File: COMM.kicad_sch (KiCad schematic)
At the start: 14 parts, among them J1 SMA Conn. (RFPC-SMA29-F), SW1 Inhibit Switch (SS5GLD2), U1 AX.25 Module (DMR818SU), U2 XBee Module (XBP9B-DMSTB002)

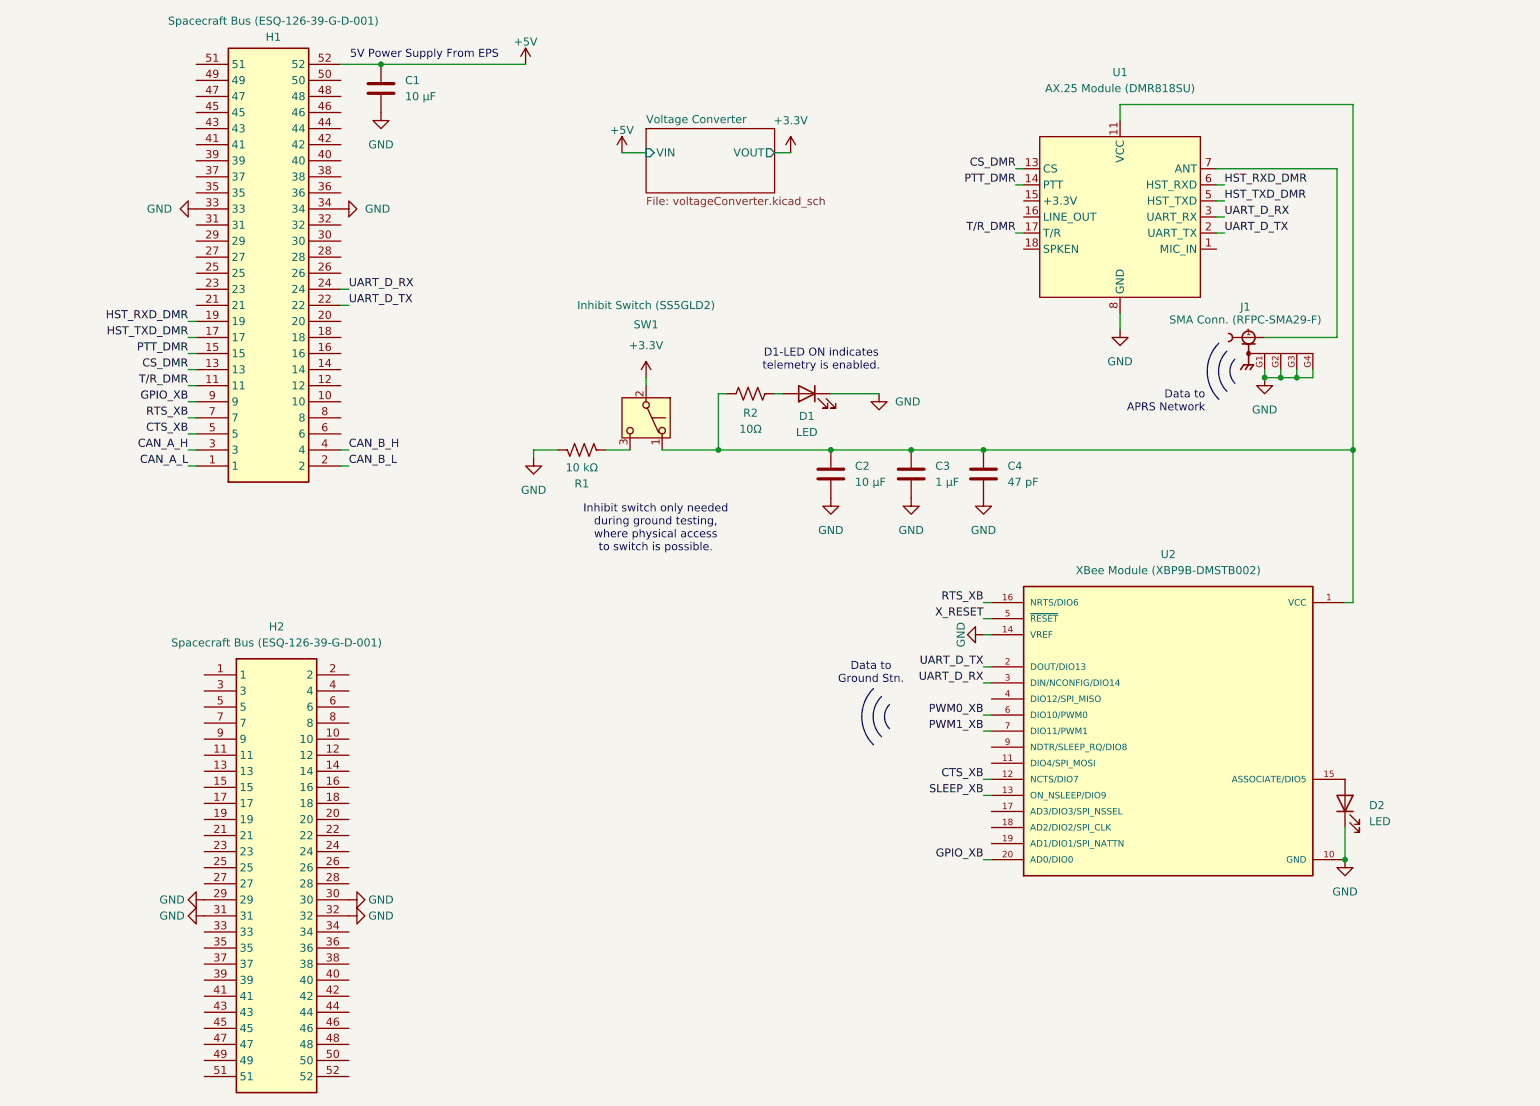
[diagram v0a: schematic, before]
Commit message: Finished schematic and fully routed PCB.
Signed-off-by: Logan Tolbert <xem6df@virginia.edu>
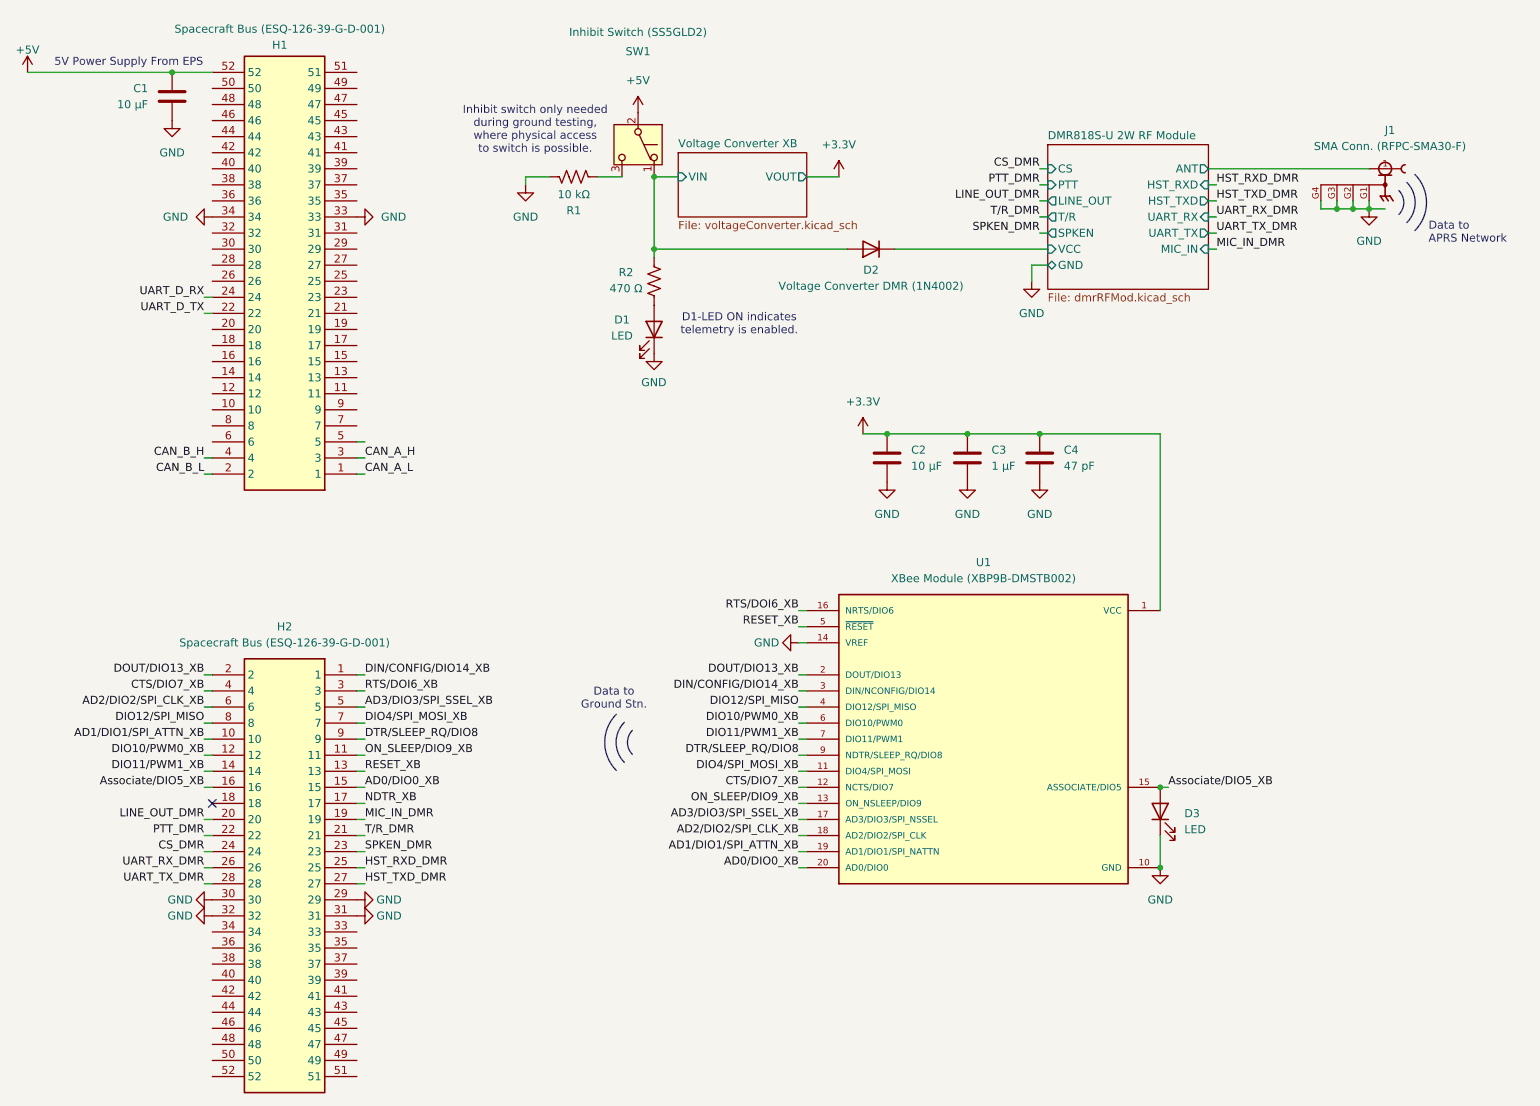
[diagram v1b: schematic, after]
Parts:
- removed J1: SMA Conn. (RFPC-SMA29-F), RFPC-SMA29-F:GRADCONN_RFPC-SMA29-F, symbol RFPC-SMA29-F:RFPC-SMA29-F
- removed U1: AX.25 Module (DMR818SU), DMR818S:DMR818SU, symbol DMR818S:DMR818S-U
- added D2: Voltage Converter DMR (1N4002), Diode_THT:D_DO-41_SOD81_P10.16mm_Horizontal, symbol Diode:1N4002
- added J1: SMA Conn. (RFPC-SMA30-F), RFPC-SMA30-F:GRADCONN_RFPC-SMA30-F, symbol RFPC-SMA30-F:RFPC-SMA30-F
- R2: value 10Ω -> 470 Ω
- renumbered D2 to D3, U2 to U1
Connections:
- net PWM0_XB is gone; now on net DIO10/PWM0_XB: U1.6 (DIO10/PWM0)
- net PWM1_XB is gone; now on net DIO11/PWM1_XB: U1.7 (DIO11/PWM1)
- net SLEEP_XB is gone; now on net ON_SLEEP/DIO9_XB: U1.13 (ON_NSLEEP/DIO9)
- net X_RESET is gone; now on net RESET_XB: U1.5 (~{RESET})
- net +3.3V: now also C2.1, C3.1, C4.1, U1.1 (VCC); no longer SW1.2 (B)
- net +5V: now also SW1.2 (B)
- net CS_DMR: now also H2.24; no longer H1.13
- net GND: now also J1.G1, J1.G2, J1.G3, J1.G4
- net HST_RXD_DMR: now also H2.25; no longer H1.19
- net HST_TXD_DMR: now also H2.27; no longer H1.17
- net PTT_DMR: now also H2.22; no longer H1.15
- net T/R_DMR: now also H2.21; no longer H1.11
- net UART_D_RX: no longer U1.3 (DIN/NCONFIG/DIO14)
- net UART_D_TX: no longer U1.2 (DOUT/DIO13)
- net DIO4/SPI_MOSI_XB: now reaches U1.11 (DIO4/SPI_MOSI)
- net DIO4/SPI_MOSI_XB: now also H2.7
- net Associate/DIO5_XB: now reaches D3.2 (A), U1.15 (ASSOCIATE/DIO5)
- net Associate/DIO5_XB: now also H2.16
- net AD3/DIO3/SPI_SSEL_XB: now reaches U1.17 (AD3/DIO3/SPI_NSSEL)
- net AD3/DIO3/SPI_SSEL_XB: now also H2.5
- net AD2/DIO2/SPI_CLK_XB: now reaches U1.18 (AD2/DIO2/SPI_CLK)
- net AD2/DIO2/SPI_CLK_XB: now also H2.6
- net AD1/DIO1/SPI_ATTN_XB: now reaches U1.19 (AD1/DIO1/SPI_NATTN)
- net AD1/DIO1/SPI_ATTN_XB: now also H2.10
- net DIO12/SPI_MISO: now reaches U1.4 (DIO12/SPI_MISO)
- net DIO12/SPI_MISO: now also H2.8
- net DTR/SLEEP_RQ/DIO8: now reaches U1.9 (NDTR/SLEEP_RQ/DIO8)
- net DTR/SLEEP_RQ/DIO8: now also H2.9
- net DIN/CONFIG/DIO14_XB: now reaches H2.1
- net DIN/CONFIG/DIO14_XB: now also U1.3 (DIN/NCONFIG/DIO14)
- net ON_SLEEP/DIO9_XB: now reaches H2.11
- net DIO10/PWM0_XB: now reaches H2.12
- net RESET_XB: now reaches H2.13
- net DIO11/PWM1_XB: now reaches H2.14
- net AD0/DIO0_XB: now reaches H2.15
- net AD0/DIO0_XB: now also U1.20 (AD0/DIO0)
- net NDTR_XB: now reaches H2.17
- net MIC_IN_DMR: now reaches H2.19
- net DOUT/DIO13_XB: now reaches H2.2
- net DOUT/DIO13_XB: now also U1.2 (DOUT/DIO13)
- net LINE_OUT_DMR: now reaches H2.20
- net SPKEN_DMR: now reaches H2.23
- net UART_RX_DMR: now reaches H2.26
- net UART_TX_DMR: now reaches H2.28
- net RTS/DOI6_XB: now reaches H2.3
- net RTS/DOI6_XB: now also U1.16 (NRTS/DIO6)
- net CTS/DIO7_XB: now reaches H2.4
- net CTS/DIO7_XB: now also U1.12 (NCTS/DIO7)
- net CTS_XB: no longer names the net of H1.5
- net CTS_XB: no longer U1.12 (NCTS/DIO7)
- net GPIO_XB: no longer names the net of H1.9
- net GPIO_XB: no longer U1.20 (AD0/DIO0)
- net RTS_XB: no longer names the net of H1.7
- net RTS_XB: no longer U1.16 (NRTS/DIO6)
- new net DMR818S-U 2W RF Module/ANT: J1.1
- new net DMR818S-U 2W RF Module/VCC: D2.1 (K)
- new net Voltage Converter XB/VIN: D2.2 (A), R2.2, SW1.1 (A)
- no-connect marks 0 -> 1
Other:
- sheet Voltage Converter renamed Voltage Converter XB
- added sheet DMR818S-U 2W RF Module (dmrRFMod.kicad_sch)
- moved on the sheet: C1, C2, C3, C4, D1, D3, H1, H2, R1, R2, SW1, U1
